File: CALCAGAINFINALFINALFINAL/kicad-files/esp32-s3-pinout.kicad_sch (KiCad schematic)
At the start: 16 parts, among them J1 Conn_01x11_Socket, J3 Micro_SD_Card, J4 FH12-24S-0.5SH_55_, SW1 SW_SPST, U1 MCP23008-xML, U8 ESP32-S3-WROOM-1

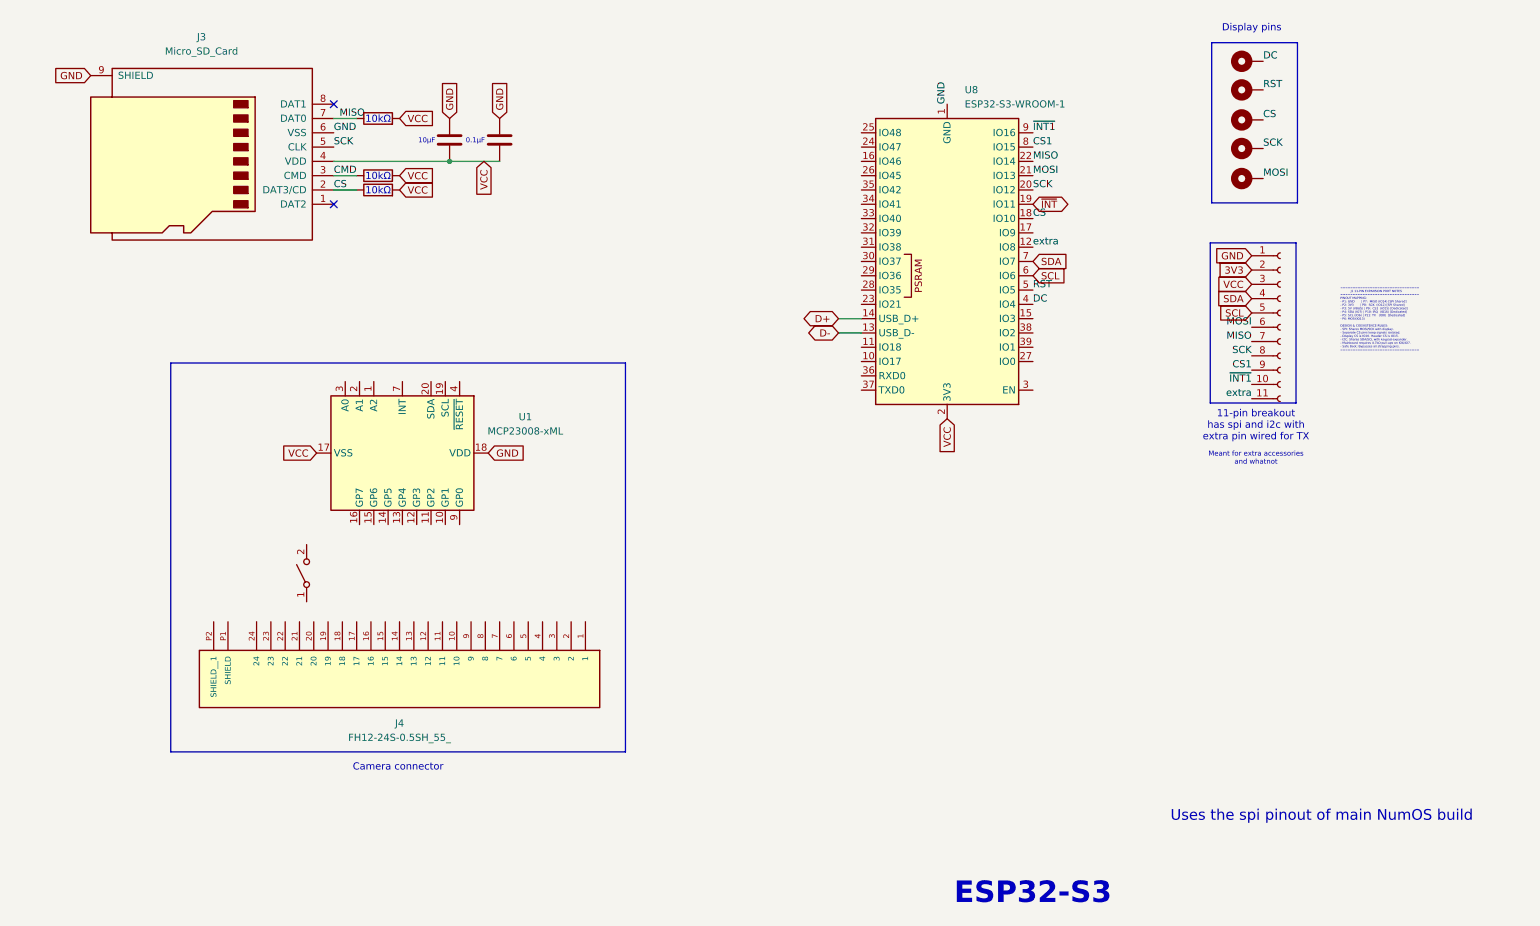
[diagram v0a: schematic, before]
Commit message: nearly finished with the no camera variant schematic stil have 2 drc warnings to fix but should be done in the next few hours.
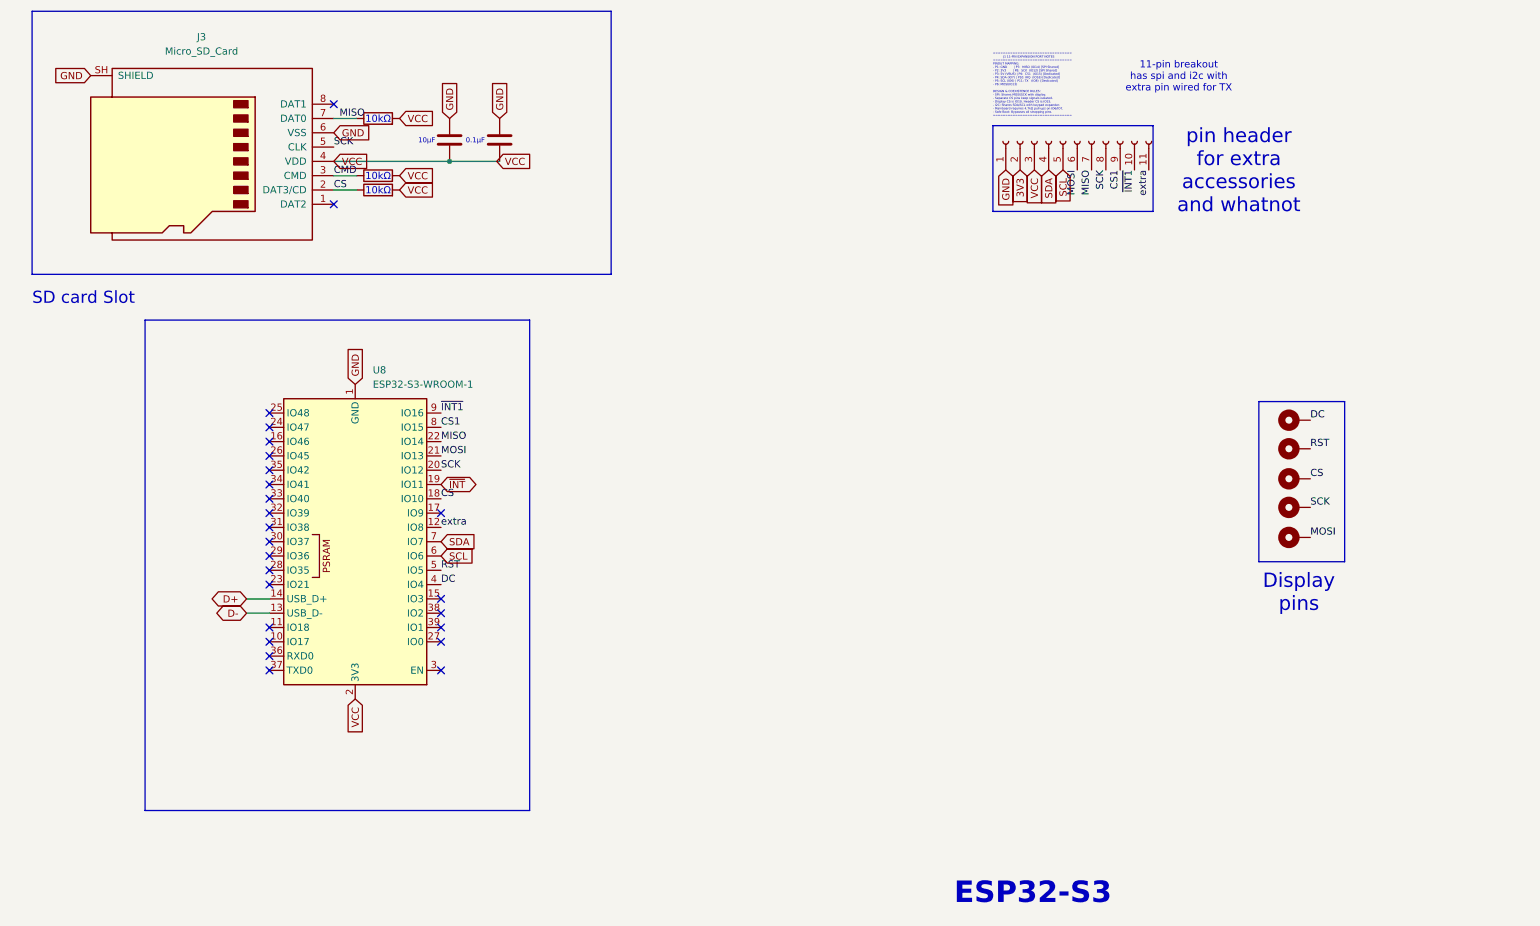
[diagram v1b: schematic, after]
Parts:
- removed J4: FH12-24S-0.5SH_55_, FH12-24S-0.5SH_55_:HRS_FH12-24S-0.5SH_55_, symbol FH12-24S-0.5SH_55_:FH12-24S-0.5SH_55_
- removed SW1: SW_SPST, symbol Switch:SW_SPST
- removed U1: MCP23008-xML, Package_DFN_QFN:QFN-20-1EP_4x4mm_P0.5mm_EP2.7x2.7mm, symbol Interface_Expansion:MCP23008-xML
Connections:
- net GND: now also J3.SH (SHIELD); no longer J3.9 (SHIELD)
- no-connect marks 2 -> 25
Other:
- note added: "SD card Slot"
- note added: "pin header for extra accessories and whatnot"
- note removed: "Camera connector"
- note removed: "Meant for extra accessories and whatnot"
- note removed: "Uses the spi pinout of main NumOS build"
- moved on the sheet: U8
